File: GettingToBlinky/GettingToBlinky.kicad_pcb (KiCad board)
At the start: 2 copper layers, 6 parts, among them U1 7555

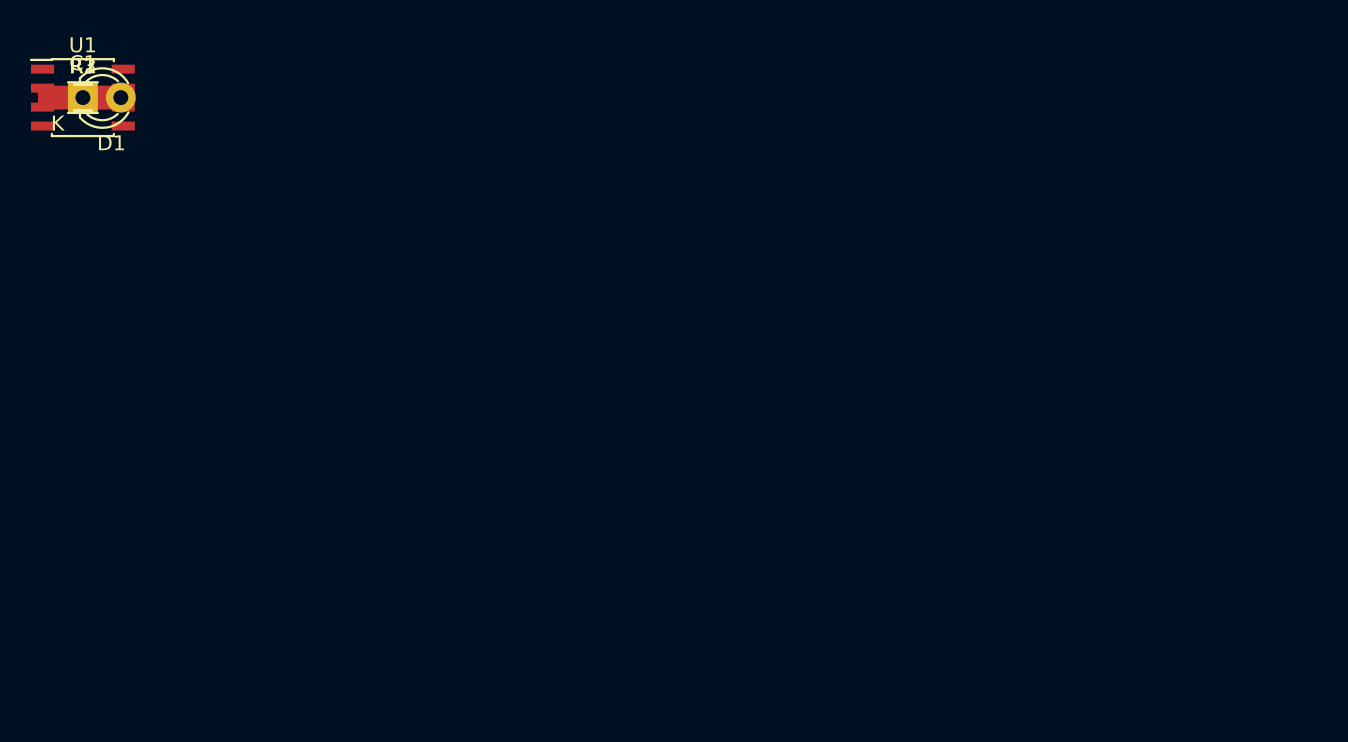
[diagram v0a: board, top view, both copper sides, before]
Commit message: finished pcb layout
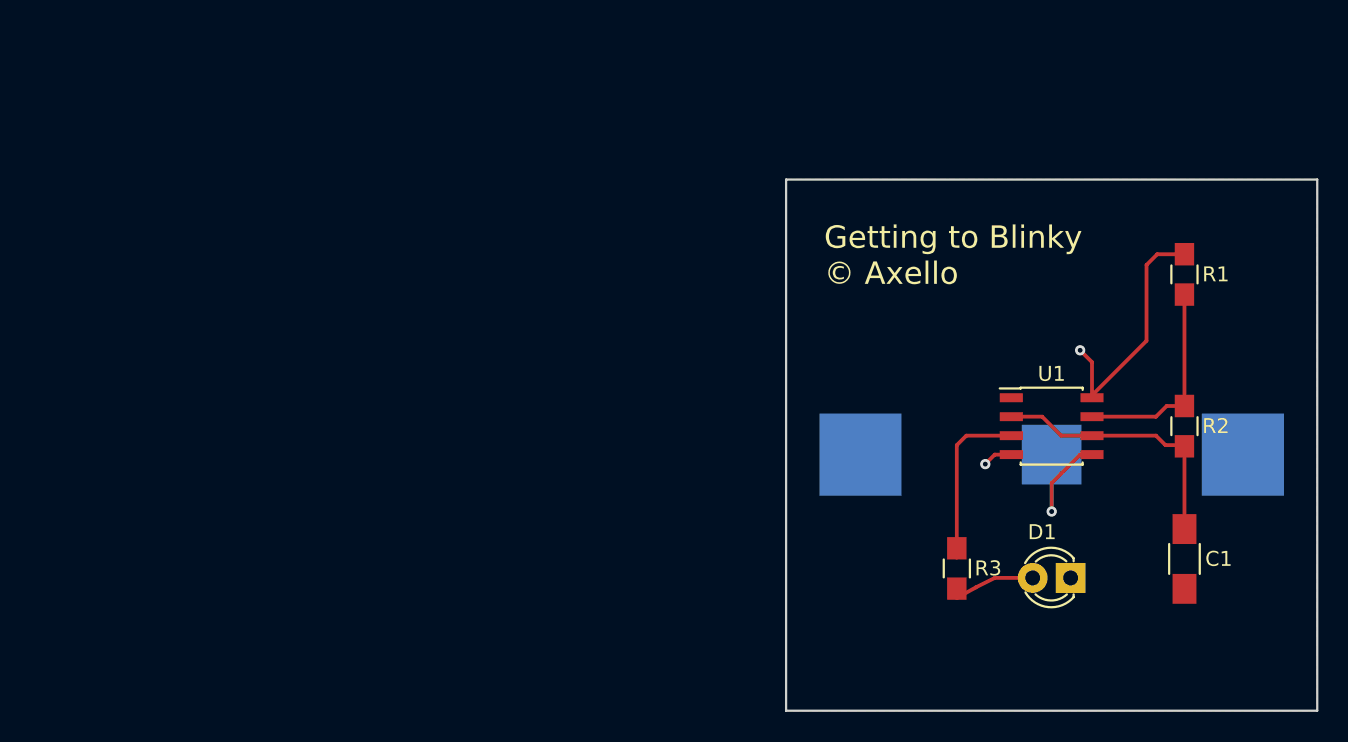
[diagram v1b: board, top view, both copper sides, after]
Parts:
- added BT1: Battery, GTB:BatteryHolder, B.Cu at (213.4, 128.9)
- moved C1 80.0 mm to (222.2, 135.9), turned to 270 degrees
- moved R2 77.0 mm to (222.2, 127.0), turned to 270 degrees
- moved R1 74.7 mm to (222.2, 116.8), turned to 270 degrees
- moved D1 73.5 mm to (214.6, 137.2), turned to 180 degrees
- moved U1 68.5 mm to (213.4, 127.0)
- moved R3 66.5 mm to (207.0, 136.5), turned to 270 degrees
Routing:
- net /VDD: track 0.00 -> 18.8 mm, vias 0 -> 2
- net Net-(C1-Pad1): track 0.00 -> 18.0 mm
- net Net-(R1-Pad2): track 0.00 -> 13.9 mm
- net Net-(R3-Pad1): track 0.00 -> 11.5 mm
- net GND: track 0.00 -> 9.20 mm, vias 0 -> 1
- net Net-(D1-Pad2): track 0.00 -> 5.42 mm
- added copper zone on B.Cu, net /VDD
- added copper zone on F.Cu, net GND
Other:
- board outline added: 35.6 x 35.6 mm
- net class Default: clearance 0.2 -> 0.254; trace_width 0.25 -> 0.254; via_dia 0.6 -> 0.6858; via_drill 0.4 -> 0.3302
- rule trace_clearance: 0.2 -> 0.254
- rule trace_min: 0.2 -> 0.1524
- rule via_min_drill: 0.3 -> 0.3302
- rule via_min_size: 0.4 -> 0.6858
- board text added: "Getting to Blinky © Axello"
